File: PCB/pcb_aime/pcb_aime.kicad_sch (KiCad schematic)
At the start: 17 parts, among them J1 Pin ESP, J2 Pin Capteur, J4 Pin LoRa, U1 LTC1050ACN8_PBF

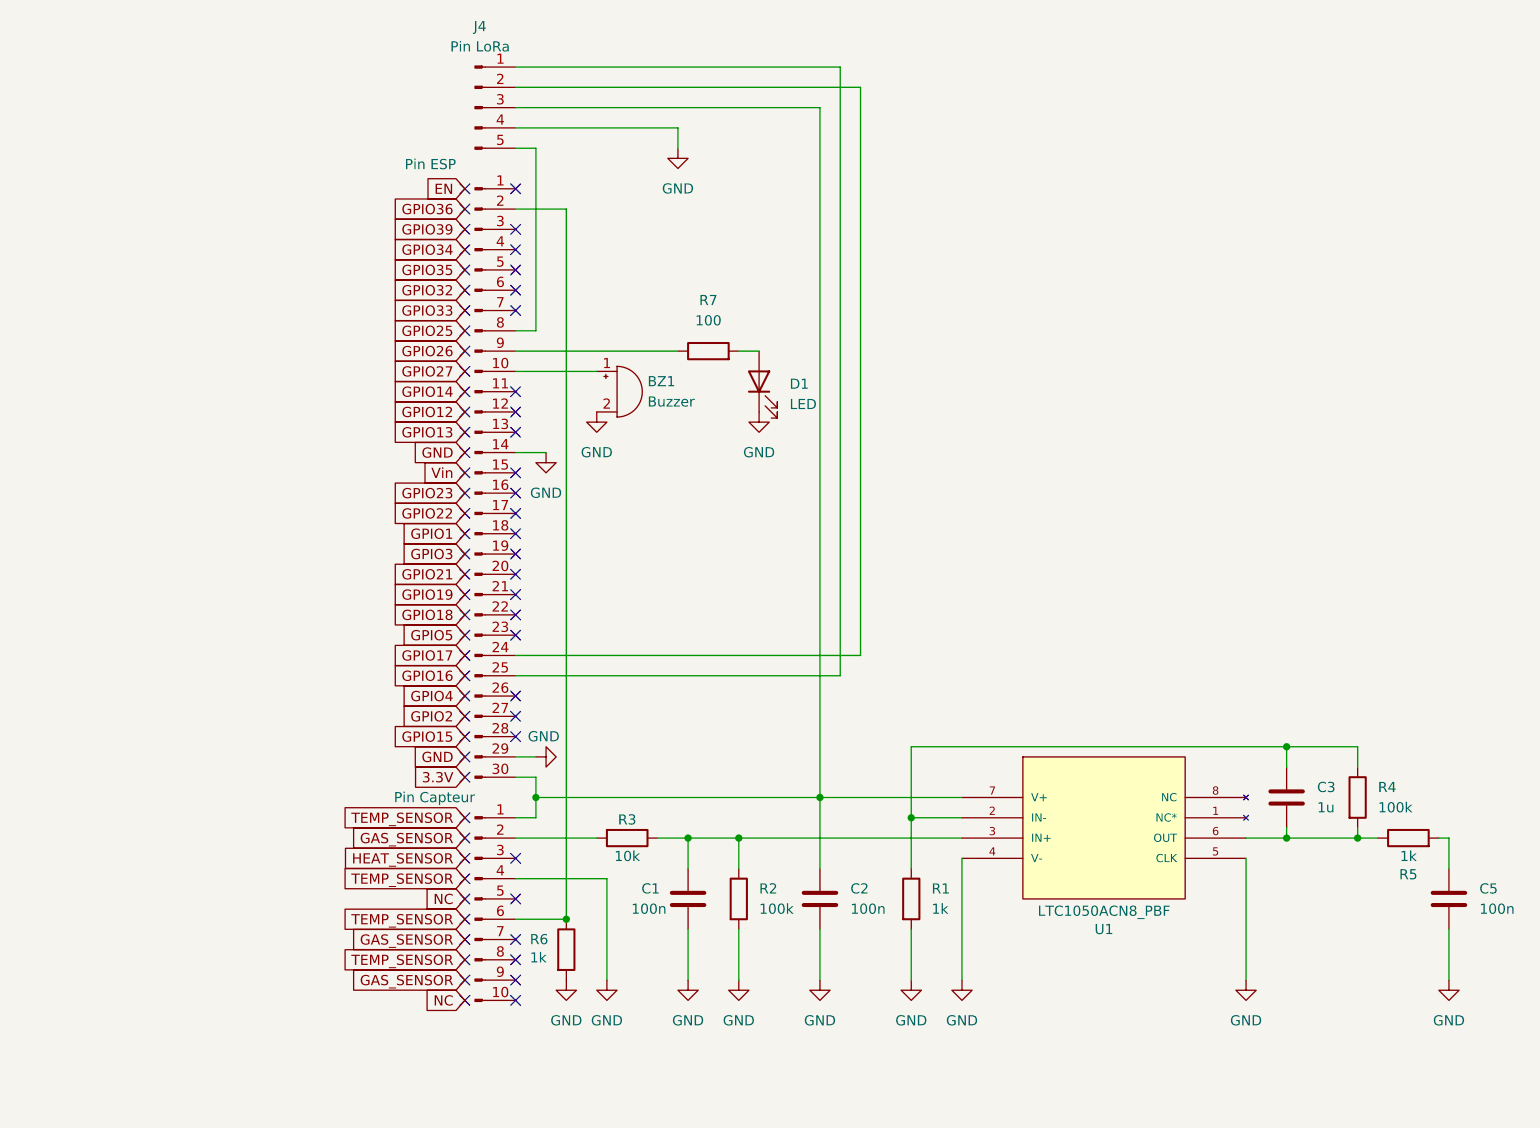
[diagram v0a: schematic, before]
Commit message: finishing some things
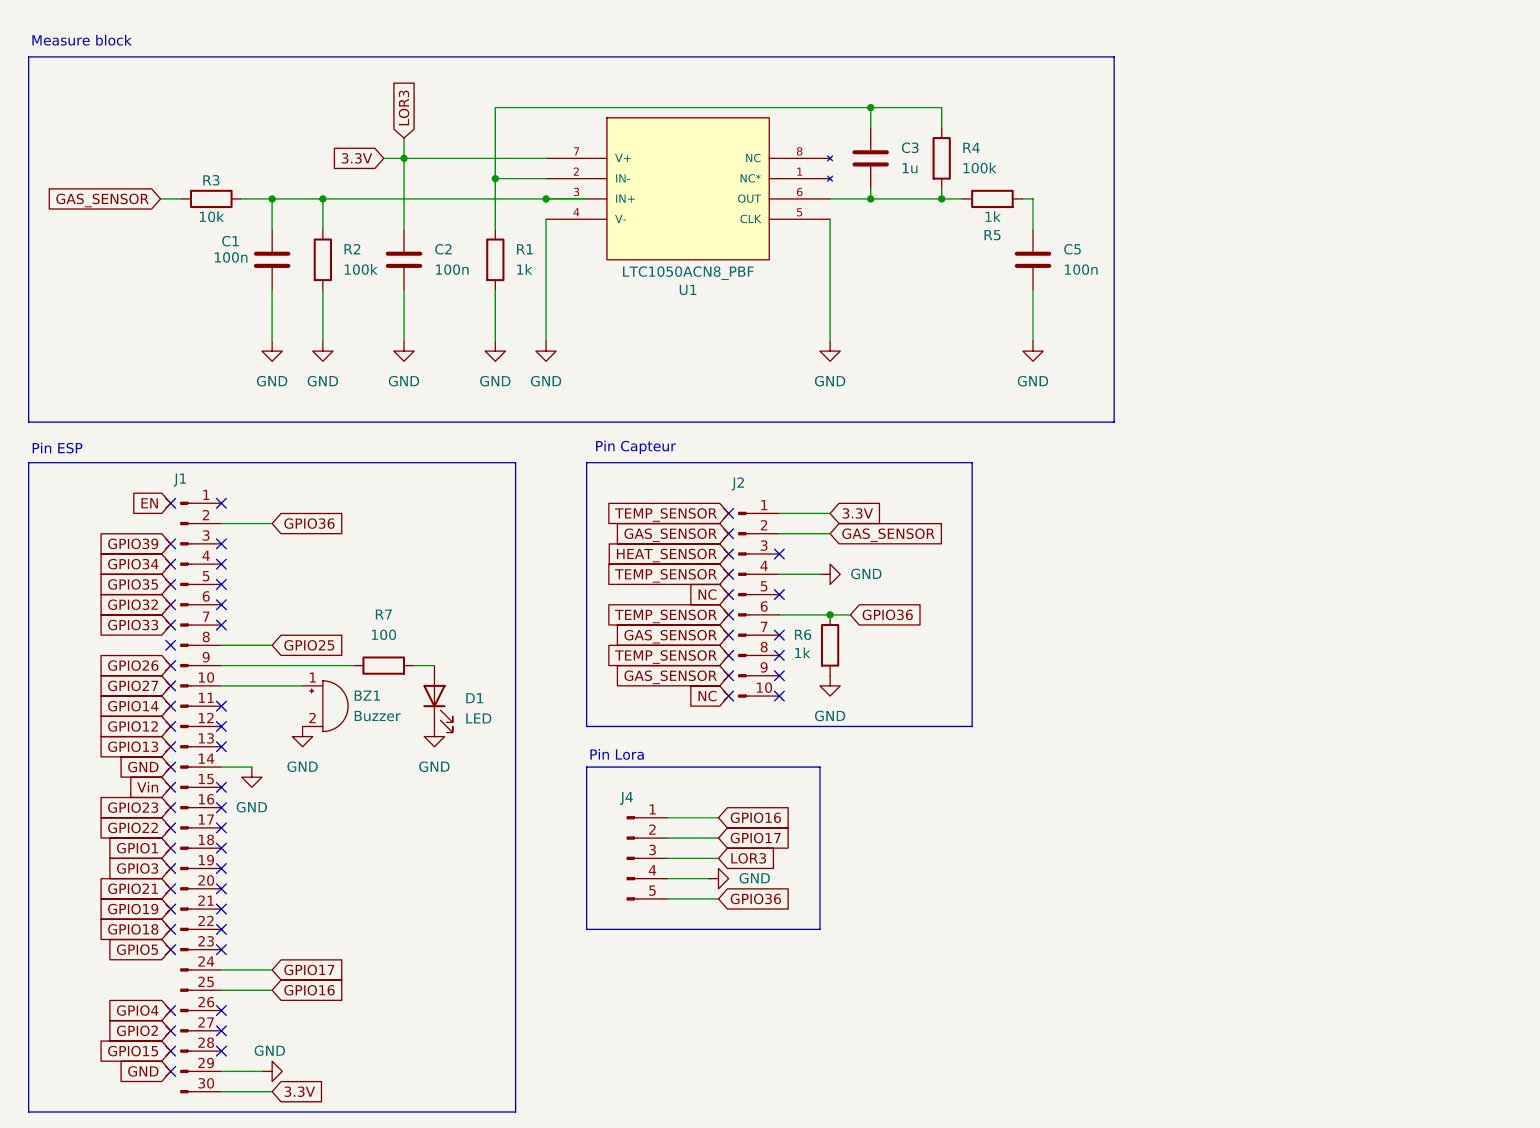
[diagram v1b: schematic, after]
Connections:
- net 3.3V: now also C2.2, J1.30 (Pin_30), J2.1 (Pin_1), J4.3 (Pin_3), U1.7 (V+)
- net GAS_SENSOR: now also J2.2 (Pin_2), R3.2
- net GPIO16: now also J1.25 (Pin_25), J4.1 (Pin_1)
- net GPIO17: now also J1.24 (Pin_24), J4.2 (Pin_2)
- net GPIO25: now also J1.8 (Pin_8)
- net GPIO36: now also J1.2 (Pin_2), J2.6 (Pin_6), J4.5 (Pin_5), R6.1
- no-connect marks 67 -> 63
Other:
- note added: "Measure block"
- note added: "Pin Capteur"
- note added: "Pin ESP"
- note added: "Pin Lora"
- moved on the sheet: BZ1, C1, C2, C3, C5, D1, J4, R1, R2, R3, R4, R5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
